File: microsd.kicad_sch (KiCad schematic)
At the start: 8 parts, among them J7 503398-1892

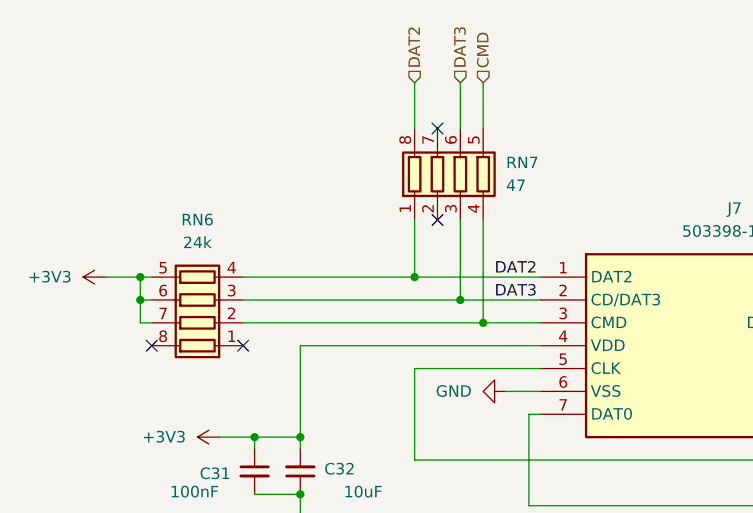
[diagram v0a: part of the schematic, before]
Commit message: Routing 06/25
Molte modifiche
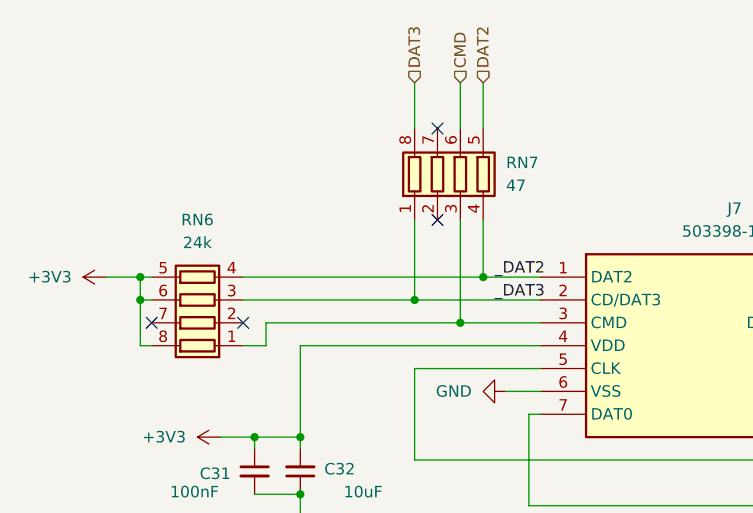
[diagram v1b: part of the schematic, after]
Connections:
- net +3V3: now also RN6.8 (R1.2); no longer RN6.7 (R2.2)
- net CMD: now also RN7.6 (R3.2); no longer RN7.5 (R4.2)
- net DAT2: now also RN7.5 (R4.2); no longer J7.1 (DAT2), RN6.4 (R4.1), RN7.1 (R1.1), RN7.8 (R1.2)
- net DAT3: now also RN7.8 (R1.2); no longer J7.2 (CD/DAT3), RN6.3 (R3.1), RN7.3 (R3.1), RN7.6 (R3.2)
- net at RN6.1 (R1.1): now also J7.3 (CMD), RN7.3 (R3.1)
- new net _DAT2: J7.1 (DAT2), RN6.4 (R4.1), RN7.4 (R4.1)
- new net _DAT3: J7.2 (CD/DAT3), RN6.3 (R3.1), RN7.1 (R1.1)
- now unconnected: RN6.2 (R2.1)
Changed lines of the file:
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@@
-	)
-	(junction
-		(at 74.93 48.26)
-		(diameter 0)
-		(color 0 0 0 0)
 	)
 	(junction
@@
 	)
 	(junction
+		(at 74.93 50.8)
+		(diameter 0)
+		(color 0 0 0 0)
+	)
+	(junction
+		(at 144.78 71.12)
+		(diameter 0)
+		(color 0 0 0 0)
+	)
+	(junction
+		(at 129.54 60.96)
+		(diameter 0)
+		(color 0 0 0 0)
+	)
+	(junction
+		(at 129.54 55.88)
+		(diameter 0)
+		(color 0 0 0 0)
+	)
+	(junction
+		(at 69.85 48.26)
+		(diameter 0)
+		(color 0 0 0 0)
+	)
+	(junction
+		(at 57.15 69.85)
+		(diameter 0)
+		(color 0 0 0 0)
+	)
+	(junction
+		(at 52.07 63.5)
+		(diameter 0)
+		(color 0 0 0 0)
+	)
+	(junction
 		(at 39.37 48.26)
 		(diameter 0)
@@
 	)
 	(junction
-		(at 144.78 71.12)
-		(diameter 0)
-		(color 0 0 0 0)
-	)
-	(junction
-		(at 129.54 60.96)
-		(diameter 0)
-		(color 0 0 0 0)
-	)
-	(junction
-		(at 69.85 45.72)
-		(diameter 0)
-		(color 0 0 0 0)
-	)
-	(junction
-		(at 129.54 55.88)
-		(diameter 0)
-		(color 0 0 0 0)
-	)
-	(junction
-		(at 57.15 69.85)
-		(diameter 0)
-		(color 0 0 0 0)
-	)
-	(junction
-		(at 52.07 63.5)
-		(diameter 0)
-		(color 0 0 0 0)
-	)
-	(junction
 		(at 39.37 45.72)
 		(diameter 0)
@@
 	)
 	(junction
-		(at 77.47 50.8)
+		(at 77.47 45.72)
 		(diameter 0)
 		(color 0 0 0 0)
@@
 	)
 	(no_connect
+		(at 40.64 50.8)
+	)
+	(no_connect
 		(at 147.32 85.09)
-	)
-	(no_connect
-		(at 50.8 53.34)
 	)
 	(no_connect
@@
 	)
 	(no_connect
+		(at 50.8 50.8)
+	)
+	(no_connect
 		(at 171.45 68.58)
-	)
-	(no_connect
-		(at 40.64 53.34)
 	)
 	(no_connect
@@
 	(wire
 		(pts
-			(xy 74.93 48.26) (xy 83.82 48.26)
-		)
-		(stroke
-			(width 0)
-			(type default)
-		)
-	)
-	(wire
-		(pts
 			(xy 129.54 60.96) (xy 130.81 60.96)
 		)
@@
 	(wire
 		(pts
+			(xy 53.34 50.8) (xy 53.34 53.34)
+		)
+		(stroke
+			(width 0)
+			(type default)
+		)
+	)
+	(wire
+		(pts
 			(xy 52.07 63.5) (xy 57.15 63.5)
 		)
@@
 	(wire
 		(pts
+			(xy 69.85 48.26) (xy 83.82 48.26)
+		)
+		(stroke
+			(width 0)
+			(type default)
+		)
+	)
+	(wire
+		(pts
 			(xy 83.82 55.88) (xy 69.85 55.88)
 		)
@@
 	(wire
 		(pts
+			(xy 74.93 39.37) (xy 74.93 50.8)
+		)
+		(stroke
+			(width 0)
+			(type default)
+		)
+	)
+	(wire
+		(pts
 			(xy 48.26 63.5) (xy 52.07 63.5)
 		)
@@
 	(wire
 		(pts
-			(xy 77.47 50.8) (xy 83.82 50.8)
+			(xy 50.8 45.72) (xy 77.47 45.72)
 		)
 		(stroke
@@
 	(wire
 		(pts
+			(xy 40.64 53.34) (xy 39.37 53.34)
+		)
+		(stroke
+			(width 0)
+			(type default)
+		)
+	)
+	(wire
+		(pts
+			(xy 74.93 50.8) (xy 83.82 50.8)
+		)
+		(stroke
+			(width 0)
+			(type default)
+		)
+	)
+	(wire
+		(pts
 			(xy 142.24 45.72) (xy 142.24 63.5)
 		)
@@
 	(wire
 		(pts
-			(xy 69.85 39.37) (xy 69.85 45.72)
-		)
-		(stroke
-			(width 0)
-			(type default)
-		)
-	)
-	(wire
-		(pts
 			(xy 83.82 60.96) (xy 82.55 60.96)
 		)
@@
 	(wire
 		(pts
+			(xy 77.47 45.72) (xy 83.82 45.72)
+		)
+		(stroke
+			(width 0)
+			(type default)
+		)
+	)
+	(wire
+		(pts
 			(xy 35.56 45.72) (xy 39.37 45.72)
 		)
@@
 	(wire
 		(pts
-			(xy 50.8 50.8) (xy 77.47 50.8)
+			(xy 77.47 39.37) (xy 77.47 45.72)
 		)
 		(stroke
@@
 	(wire
 		(pts
-			(xy 50.8 48.26) (xy 74.93 48.26)
+			(xy 50.8 48.26) (xy 69.85 48.26)
 		)
 		(stroke
@@
 	(wire
 		(pts
-			(xy 39.37 48.26) (xy 39.37 50.8)
-		)
-		(stroke
-			(width 0)
-			(type default)
-		)
-	)
-	(wire
-		(pts
 			(xy 144.78 88.9) (xy 149.86 88.9)
 		)
@@
 	(wire
 		(pts
-			(xy 77.47 39.37) (xy 77.47 50.8)
-		)
-		(stroke
-			(width 0)
-			(type default)
-		)
-	)
-	(wire
-		(pts
 			(xy 57.15 53.34) (xy 83.82 53.34)
 		)
@@
 	(wire
 		(pts
-			(xy 39.37 50.8) (xy 40.64 50.8)
+			(xy 53.34 50.8) (xy 74.93 50.8)
 		)
 		(stroke
@@
 	(wire
 		(pts
-			(xy 69.85 45.72) (xy 83.82 45.72)
-		)
-		(stroke
-			(width 0)
-			(type default)
-		)
-	)
-	(wire
-		(pts
 			(xy 171.45 63.5) (xy 176.53 63.5)
 		)
@@
 	(wire
 		(pts
-			(xy 50.8 45.72) (xy 69.85 45.72)
+			(xy 53.34 53.34) (xy 50.8 53.34)
 		)
 		(stroke
@@
 	(wire
 		(pts
+			(xy 69.85 39.37) (xy 69.85 48.26)
+		)
+		(stroke
+			(width 0)
+			(type default)
+		)
+	)
+	(wire
+		(pts
 			(xy 153.67 48.26) (xy 153.67 50.8)
 		)
@@
 	(wire
 		(pts
-			(xy 74.93 39.37) (xy 74.93 48.26)
-		)
-		(stroke
-			(width 0)
-			(type default)
-		)
-	)
-	(wire
-		(pts
 			(xy 149.86 63.5) (xy 161.29 63.5)
 		)
@@
 	(wire
 		(pts
+			(xy 39.37 53.34) (xy 39.37 48.26)
+		)
+		(stroke
+			(width 0)
+			(type default)
+		)
+	)
+	(wire
+		(pts
 			(xy 57.15 63.5) (xy 57.15 64.77)
 		)
@@
 		)
 	)
-	(label "DAT3"
+	(label "_DAT3"
 		(at 78.74 48.26 0)
 		(effects
@@
 		)
 	)
-	(label "DAT2"
+	(label "_DAT2"
 		(at 78.74 45.72 0)
 		(effects
@@
 			)
 			(justify left bottom)
+		)
+	)
+	(hierarchical_label "DAT3"
+		(shape input)
+		(at 69.85 24.13 90)
+		(effects
+			(font
+				(size 1.27 1.27)
+			)
+			(justify left)
 		)
 	)
@@
 	(hierarchical_label "DAT2"
 		(shape input)
-		(at 69.85 24.13 90)
+		(at 77.47 24.13 90)
+		(effects
+			(font
+				(size 1.27 1.27)
+			)
+			(justify left)
+		)
+	)
+	(hierarchical_label "CMD"
+		(shape input)
+		(at 74.93 24.13 90)
 		(effects
 			(font
@@
 		)
 	)
-	(hierarchical_label "DAT3"
-		(shape input)
-		(at 74.93 24.13 90)
-		(effects
-			(font
-				(size 1.27 1.27)
-			)
-			(justify left)
-		)
-	)
 	(hierarchical_label "DAT1"
 		(shape input)
@@
 		(effects
 			(font
-				(size 1.27 1.27)
-			)
-			(justify left)
-		)
-	)
-	(hierarchical_label "CMD"
-		(shape input)
-		(at 77.47 24.13 90)
-		(effects
-			(font

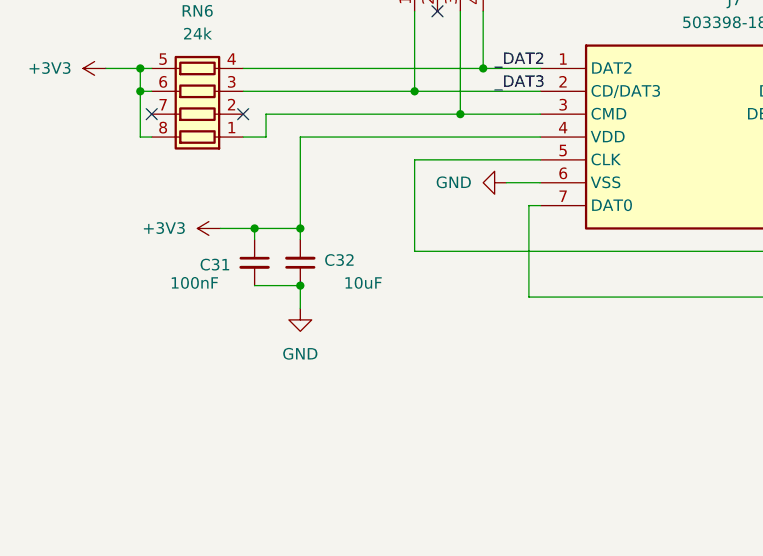
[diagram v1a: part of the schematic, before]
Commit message: Names fix
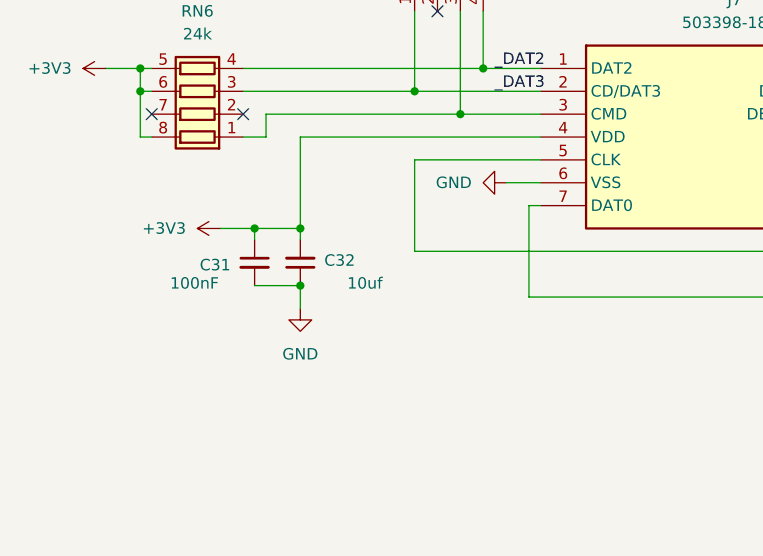
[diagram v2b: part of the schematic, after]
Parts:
- C32: value 10uF -> 10uf
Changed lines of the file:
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@@
 			)
 		)
-		(property "Value" "10uF"
+		(property "Value" "10uf"
 			(at 66.294 69.596 0)
 			(effects
